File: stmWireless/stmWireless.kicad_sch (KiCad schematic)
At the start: 31 parts, among them J1 SWD, J2 CORTEX_DEBUG, J3 Conn_02x08_Top_Bottom, U1 STM32WLE5CBU6, U2 AP63203WU, Y1 Crystal_32MHz, Y2 Crystal_32.768kHz

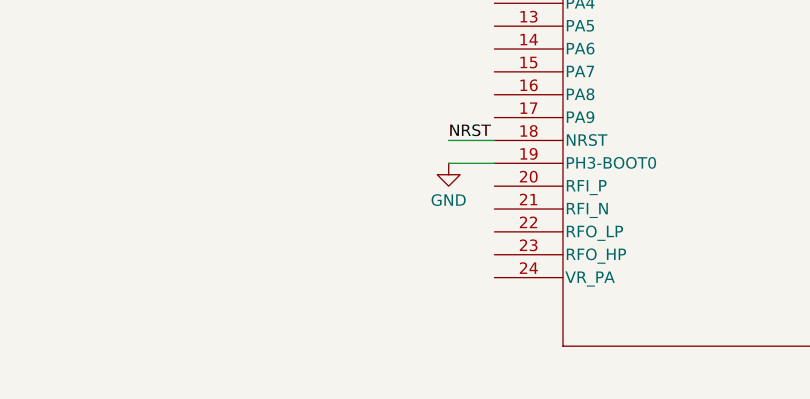
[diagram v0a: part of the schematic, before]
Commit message: begining of wireless thing
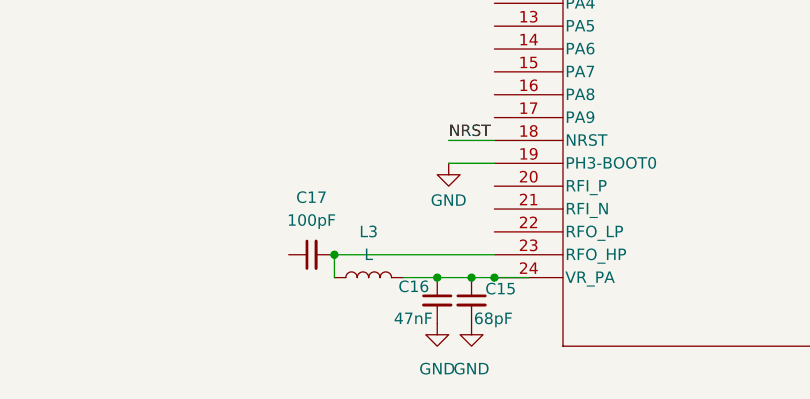
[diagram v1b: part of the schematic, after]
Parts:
- added C15: 68pF, symbol Device:C_Small
- added C16: 47nF, symbol Device:C_Small
- added C17: 100pF, symbol Device:C_Small
- added L3: L, symbol Device:L
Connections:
- net GND: now also C15.2, C16.2
- net at U1.23 (RFO_HP): now also C17.2, L3.1
- net at U1.24 (VR_PA): now also C15.1, C16.1, L3.2
